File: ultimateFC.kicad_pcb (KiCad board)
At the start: 6 copper layers, 36 x 36 mm, 227 parts, among them J1 USB_B_Micro, J2 Conn_Coaxial, J3 Conn_Coaxial, J4 Conn_Coaxial, J5 Conn_Coaxial, J8 Conn_Coaxial, J9 Conn_Coaxial, SW1 SW_Push, U1 LMR33630CQRNX, U2 TPS62824ADMQ, U3 LMR33620CRNXT, U4 S25FL064L, U5 DPS310, U6 BMI270, U7 STM32H735VGH6, U8 ICM-20602, Y1 CSTNE8M00G550000R0

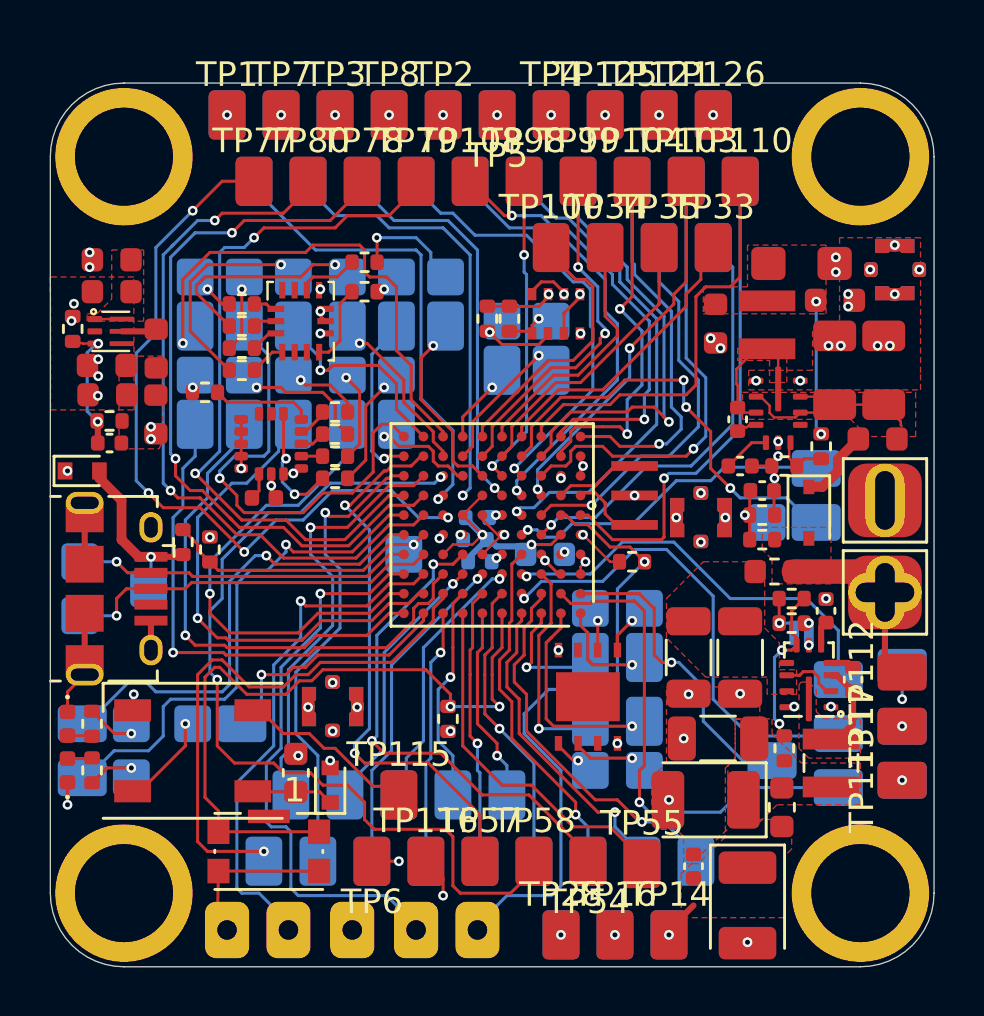
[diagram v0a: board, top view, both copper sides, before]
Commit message: update layout
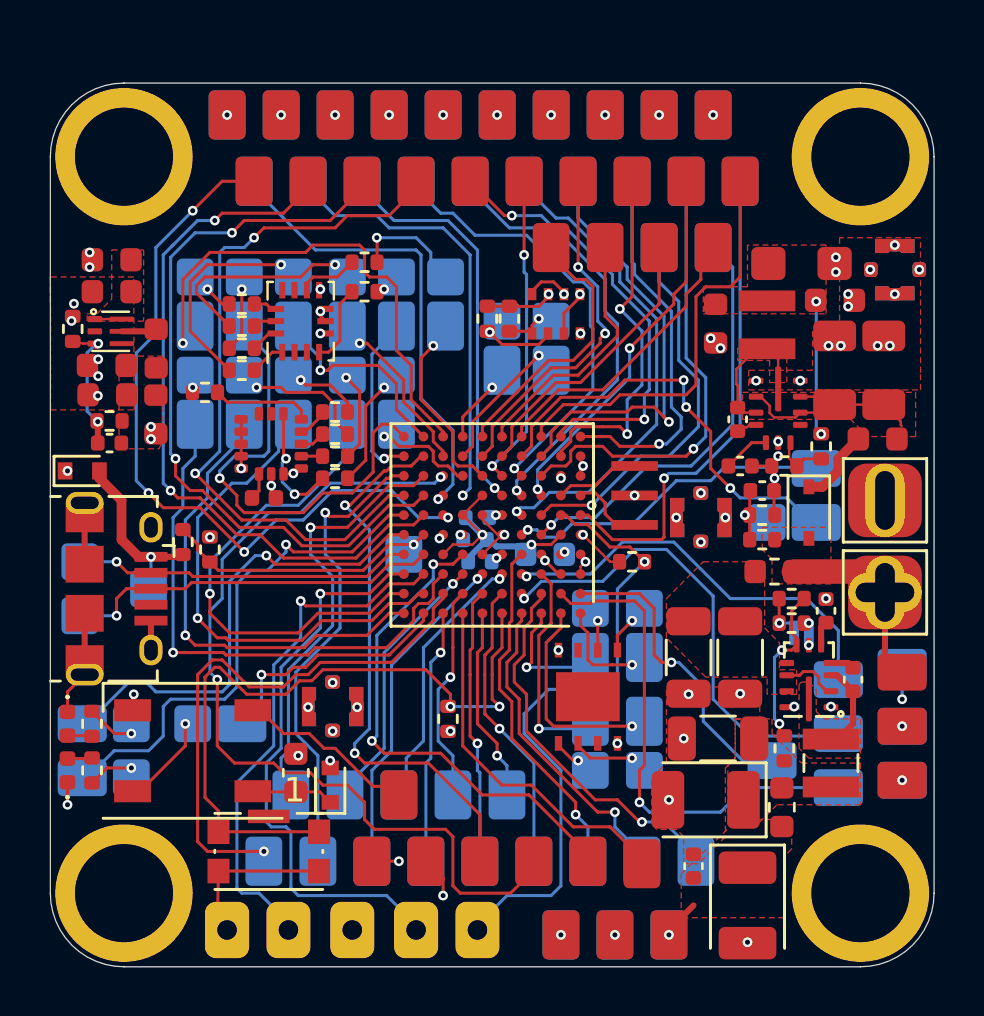
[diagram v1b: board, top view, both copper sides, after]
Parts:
- TP141: moved to F.Cu
- TP65, TP67, TP88, TP89: moved to B.Cu
- turned TP141 to 0 degrees
- turned TP65 to 180 degrees
- turned TP67 to 180 degrees
- turned TP88 to 180 degrees
- turned TP89 to 180 degrees
